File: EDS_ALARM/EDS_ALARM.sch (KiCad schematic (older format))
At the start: 28 parts, among them J1 USB_B_Micro, J2 Conn_01x06_Male, J3 73412-0110, SW1 SW_Push, U1 EKMC1601111, U2 CMWX1ZZABZ-078, U3 LT1117-3.3, U4 TGS2611-E00

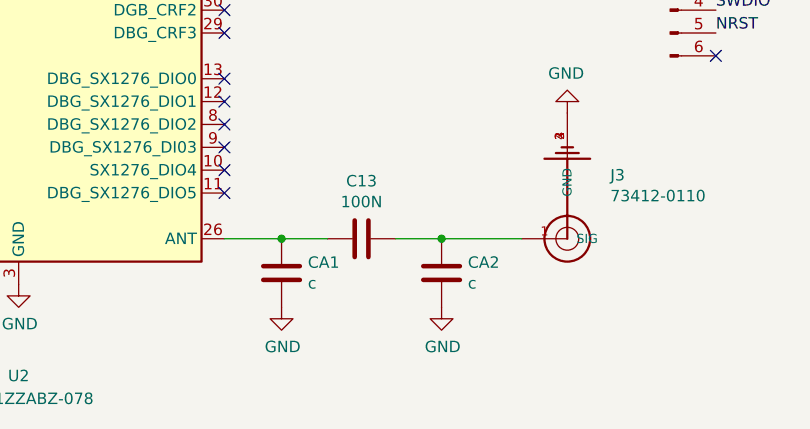
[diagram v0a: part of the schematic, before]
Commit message: a
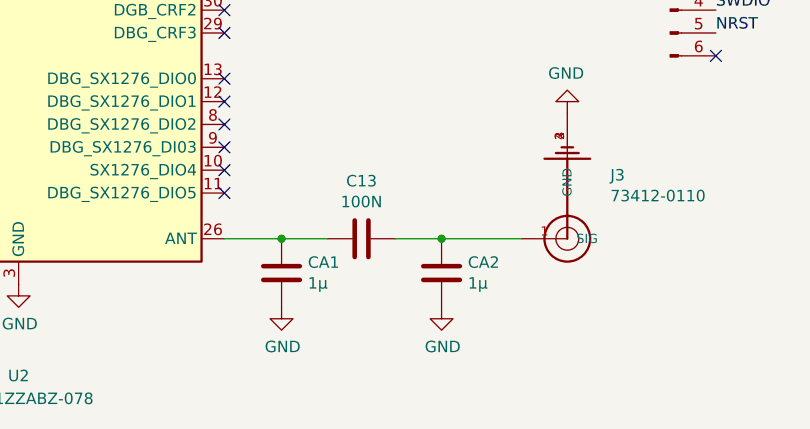
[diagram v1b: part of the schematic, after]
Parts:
- CA1, CA2: value c -> 1µ
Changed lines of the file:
@@
 P 4950 6500
 F 0 "CA1" H 5065 6546 50  0000 L CNN
-F 1 "c" H 5065 6455 50  0000 L CNN
+F 1 "1µ" H 5065 6455 50  0000 L CNN
 F 2 "Capacitor_SMD:C_0805_2012Metric_Pad1.15x1.40mm_HandSolder" H 4988 6350 50  0001 C CNN
 F 3 "~" H 4950 6500 50  0001 C CNN
@@
 P 5650 6500
 F 0 "CA2" H 5765 6546 50  0000 L CNN
-F 1 "c" H 5765 6455 50  0000 L CNN
+F 1 "1µ" H 5765 6455 50  0000 L CNN
 F 2 "Capacitor_SMD:C_0805_2012Metric_Pad1.15x1.40mm_HandSolder" H 5688 6350 50  0001 C CNN
 F 3 "~" H 5650 6500 50  0001 C CNN

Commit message: s
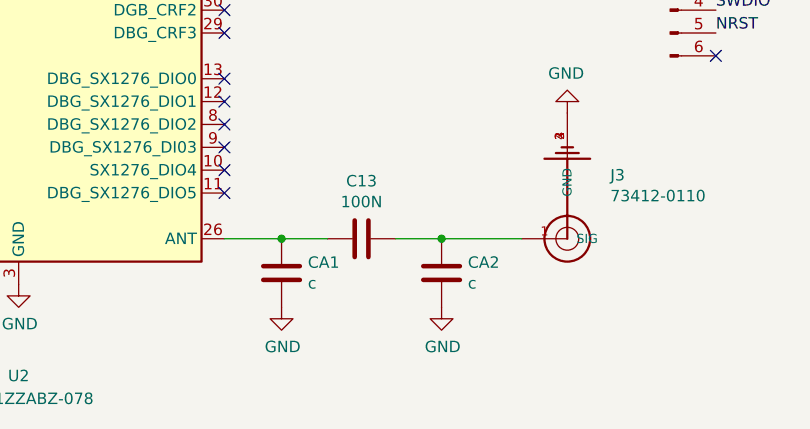
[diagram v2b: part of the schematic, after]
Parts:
- CA1, CA2: value 1µ -> c
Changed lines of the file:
@@
 P 4950 6500
 F 0 "CA1" H 5065 6546 50  0000 L CNN
-F 1 "1µ" H 5065 6455 50  0000 L CNN
+F 1 "c" H 5065 6455 50  0000 L CNN
 F 2 "Capacitor_SMD:C_0805_2012Metric_Pad1.15x1.40mm_HandSolder" H 4988 6350 50  0001 C CNN
 F 3 "~" H 4950 6500 50  0001 C CNN
@@
 P 5650 6500
 F 0 "CA2" H 5765 6546 50  0000 L CNN
-F 1 "1µ" H 5765 6455 50  0000 L CNN
+F 1 "c" H 5765 6455 50  0000 L CNN
 F 2 "Capacitor_SMD:C_0805_2012Metric_Pad1.15x1.40mm_HandSolder" H 5688 6350 50  0001 C CNN
 F 3 "~" H 5650 6500 50  0001 C CNN
